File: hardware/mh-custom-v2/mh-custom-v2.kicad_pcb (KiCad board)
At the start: 2 copper layers, 99.1 x 99.1 mm, 106 parts, among them J1 Conn_01x03_Male, J3 Conn_02x19_Top_Bottom, J4 Conn_02x19_Top_Bottom, J5 Screw_Terminal_01x04, J6 Screw_Terminal_01x04, J7 Screw_Terminal_01x04, J8 Screw_Terminal_01x04, SW1 SW_DIP_x04, T1 AO3400A, T2 AO3400A, T3 AO3400A, T4 AO3400A, T5 AO3400A, U2 ADE7953xCP, Y1 3.58MHz

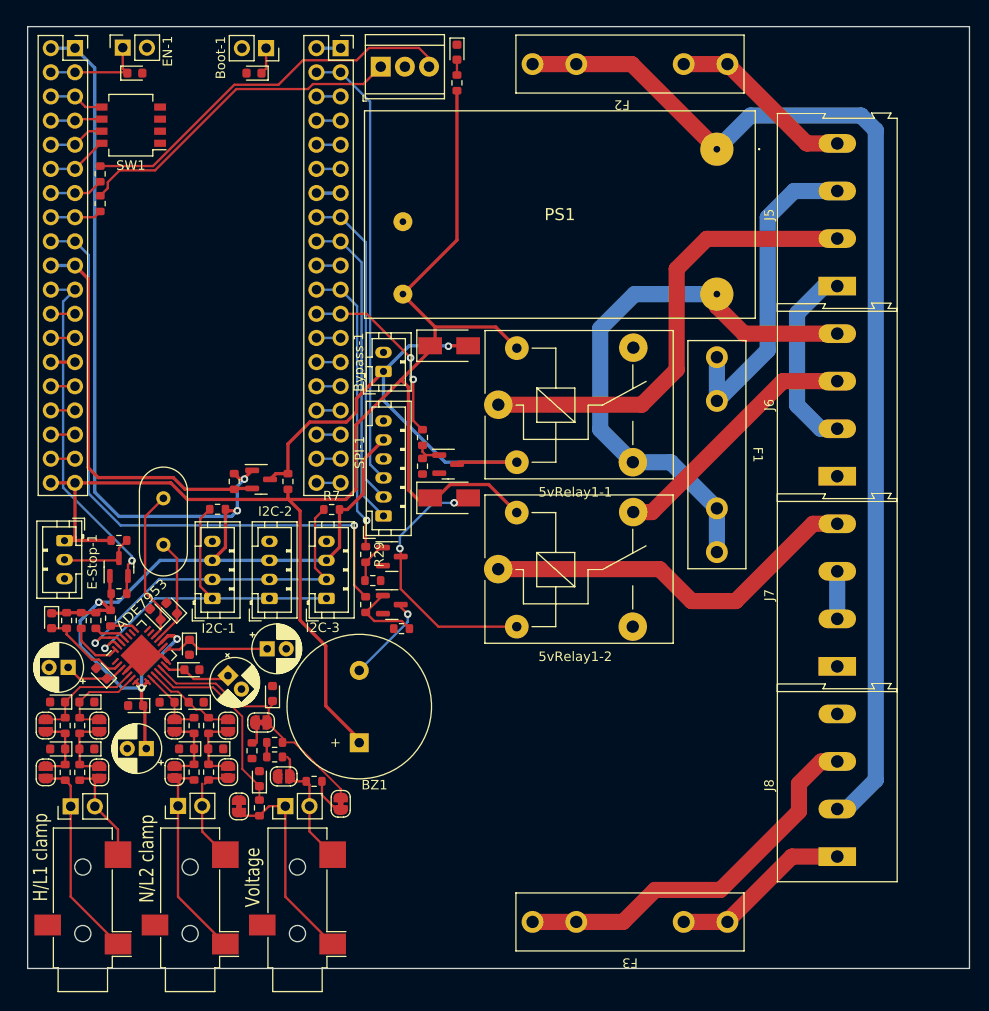
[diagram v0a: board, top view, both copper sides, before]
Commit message: approaching ordering from JLCPCB
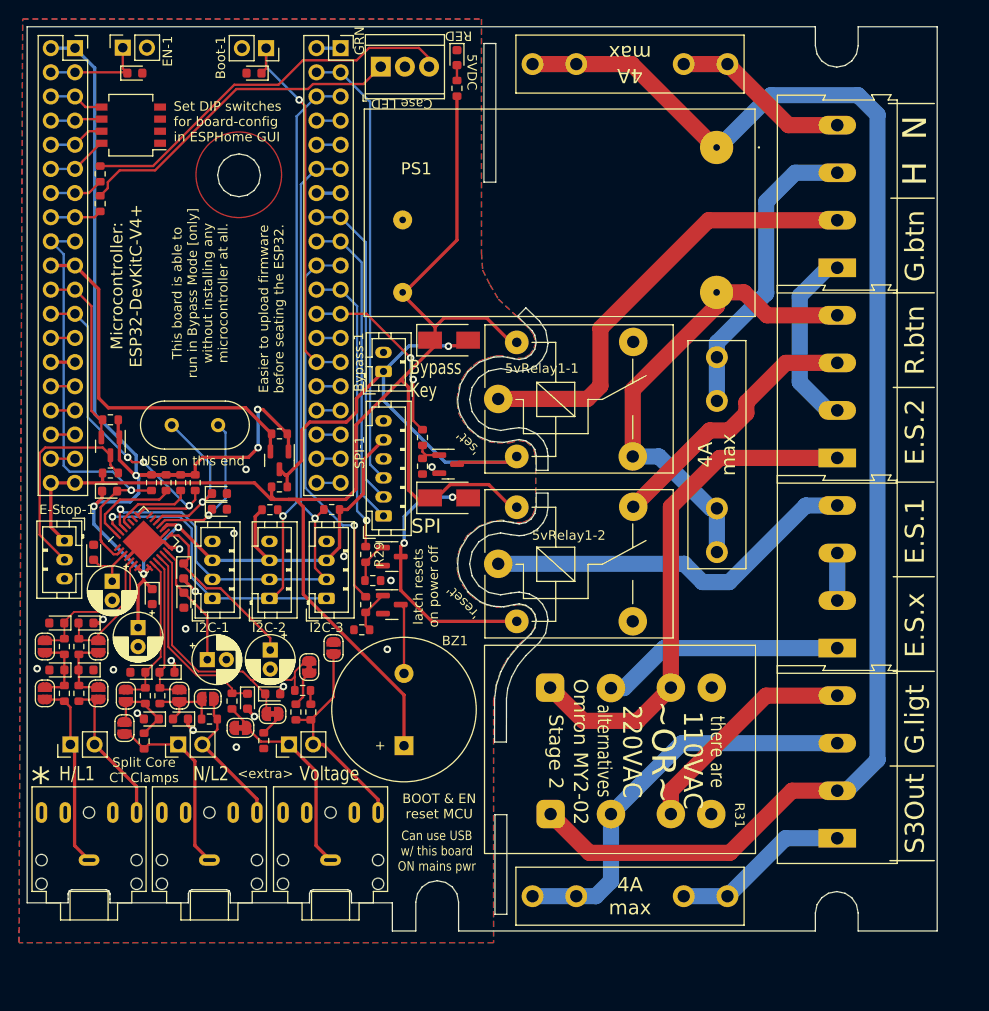
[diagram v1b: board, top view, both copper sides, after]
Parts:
- added R31: Relay_Omron_MY2-02, MY2-02 AC110 Omron:relay-Omron-MY2-02, F.Cu at (96.3, 99.1)
- IN-1, IN-2, IN-3: footprint Connector_Audio:Jack_3.5mm_CUI_SJ-3523-SMT_Horizontal -> Connector_Audio:Jack_3.5mm_CUI_SJ1-3525N_Horizontal
- moved R3 18.3 mm to (41.7, 64.2), turned to 0 degrees
- moved R22 17.0 mm to (46.0, 70.8)
- moved R24 17.0 mm to (47.6, 70.8)
- moved R25 17.0 mm to (49.1, 70.8)
- moved R23 16.8 mm to (50.6, 70.8)
- moved C15 14.9 mm to (41.6, 71.7), turned to 0 degrees
- moved JP7 14.8 mm to (62.6, 90.2)
- moved JP1 14.5 mm to (65.2, 88.2), turned to -90 degrees
- moved C20 14.4 mm to (53.2, 72.0), turned to 0 degrees
- moved Y1 13.8 mm to (53.1, 64.8), turned to 180 degrees
- moved C16 12.8 mm to (40.0, 78.2), turned to 90 degrees
- moved C14 12.7 mm to (44.6, 86.1), turned to -90 degrees
- moved T2 12.7 mm to (41.7, 67.0), turned to -90 degrees
- moved U2 12.0 mm to (45.2, 77.0)
- moved R20 11.6 mm to (54.5, 93.8)
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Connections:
- J3 pad 17: buzz -> ade7953-reset
- J3 pad 18: buzz -> ade7953-reset
- J4 pad 19: ade7953-reset -> buzz
- J4 pad 20: ade7953-reset -> buzz
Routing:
- net Member-E-Stop-sw2-2: track 0.00 -> 54.2 mm
- net SCL: track 40.3 -> 89.5 mm, vias 1 -> 2
- net SDA: track 41.2 -> 78.0 mm, vias 1 -> 2
- net mains-fused-N/L2: track 115.6 -> 151.2 mm
- net ade7953-reset: track 11.9 -> 47.5 mm, vias 0 -> 1
- net boot: track 5.36 -> 40.6 mm, vias 0 -> 1
- net ade7953-IRQ: track 5.34 -> 36.2 mm, vias 0 -> 3
- net buzz: track 67.0 -> 41.2 mm
- net Member-E-Stop-aux-2: track 0.00 -> 25.5 mm
- net Green-Indicator-light-1: track 0.00 -> 24.1 mm
- net read-E-Stop: track 38.3 -> 19.5 mm, vias 1 -> 0
- net Net-(E-Stop-1-Pad2): track 8.06 -> 22.5 mm
- net GND: track 16.2 -> 25.7 mm, vias 0 -> 18
- net VP_IN: track 13.4 -> 22.7 mm
- net IBP: track 7.48 -> 16.1 mm
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- added copper zone on B.Cu, net GND
- added copper zone on F.Cu, net GND
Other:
- board size 99.1 x 99.1 mm -> 95.7 x 95.1 mm
- board text added: "'reset'"
- board text added: "'set'"
- board text added: "*"
- board text added: "4A max"
- board text added: "5VDC"
- board text added: "<extra>"
- board text added: "BOOT & EN reset MCU"
- board text added: "Bypass Key"
- board text added: "Can use USB w/ this board ON mains pwr"
- board text added: "Case LED"
- board text added: "Designed by: Corey Rice, Iris Artin, Vincent, Lior, J.R."
- board text added: "E.S.1"
- board text added: "E.S.2"
- board text added: "E.S.x"
- board text added: "Easier to upload firmware before seating the ESP32."
- board text added: "G.btn"
- board text added: "G.ligt"
- board text added: "GRN"
- board text added: "H"
- board text added: "H/L1"
- board text added: "Hardware: V1.2.0"
- board text added: "Keep fingers out of High Voltage Area"
- board text added: "Microcontroller: ESP32-DevKitC-V4+"
- board text added: "N"
- board text added: "N/L2"
- board text added: "R.btn"
- board text added: "RED"
- board text added: "S3Out"
- board text added: "SPI"
- board text added: "Set DIP switches for board-config in ESPHome GUI"
- board text added: "Split Core CT Clamps"
- board text added: "This board is able to run in Bypass Mode [only] without installing any microcontroller at all."
- board text added: "USB on this end"
- board text added: "latch resets on power off"
- board text added: "makehaven.org/toolauth"
- board text removed: "ADE7953"
- board text removed: "H/L1 clamp"
- board text removed: "N/L2 clamp"
